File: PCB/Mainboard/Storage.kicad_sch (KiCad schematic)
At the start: 2 parts, among them U41 SDBL-4, U42 SC414281PU4

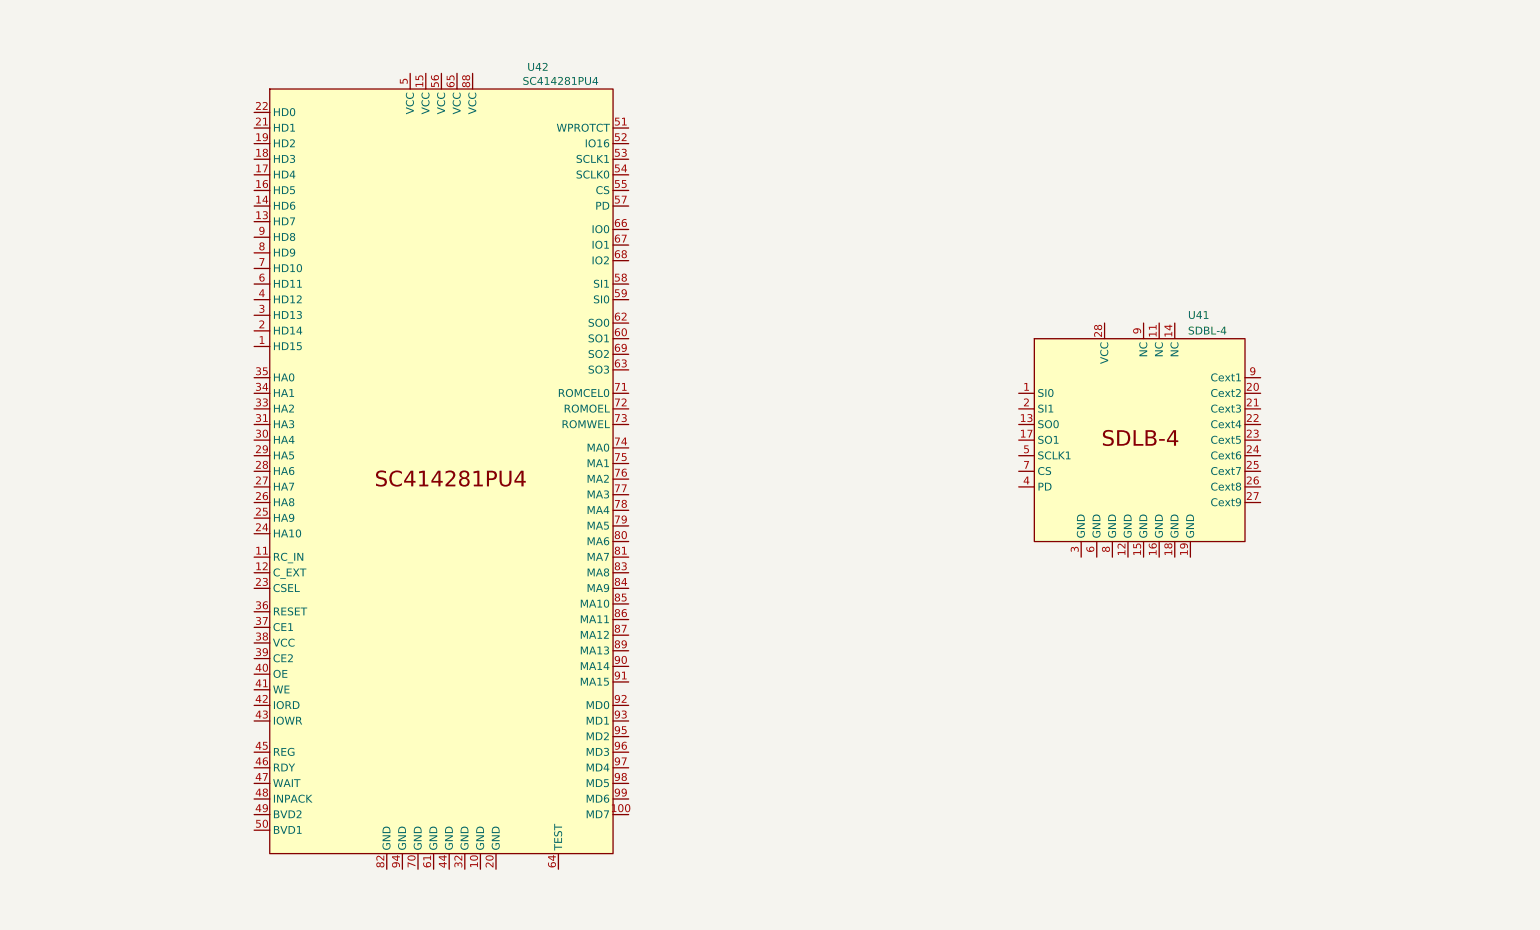
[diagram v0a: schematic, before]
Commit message: Add files via upload
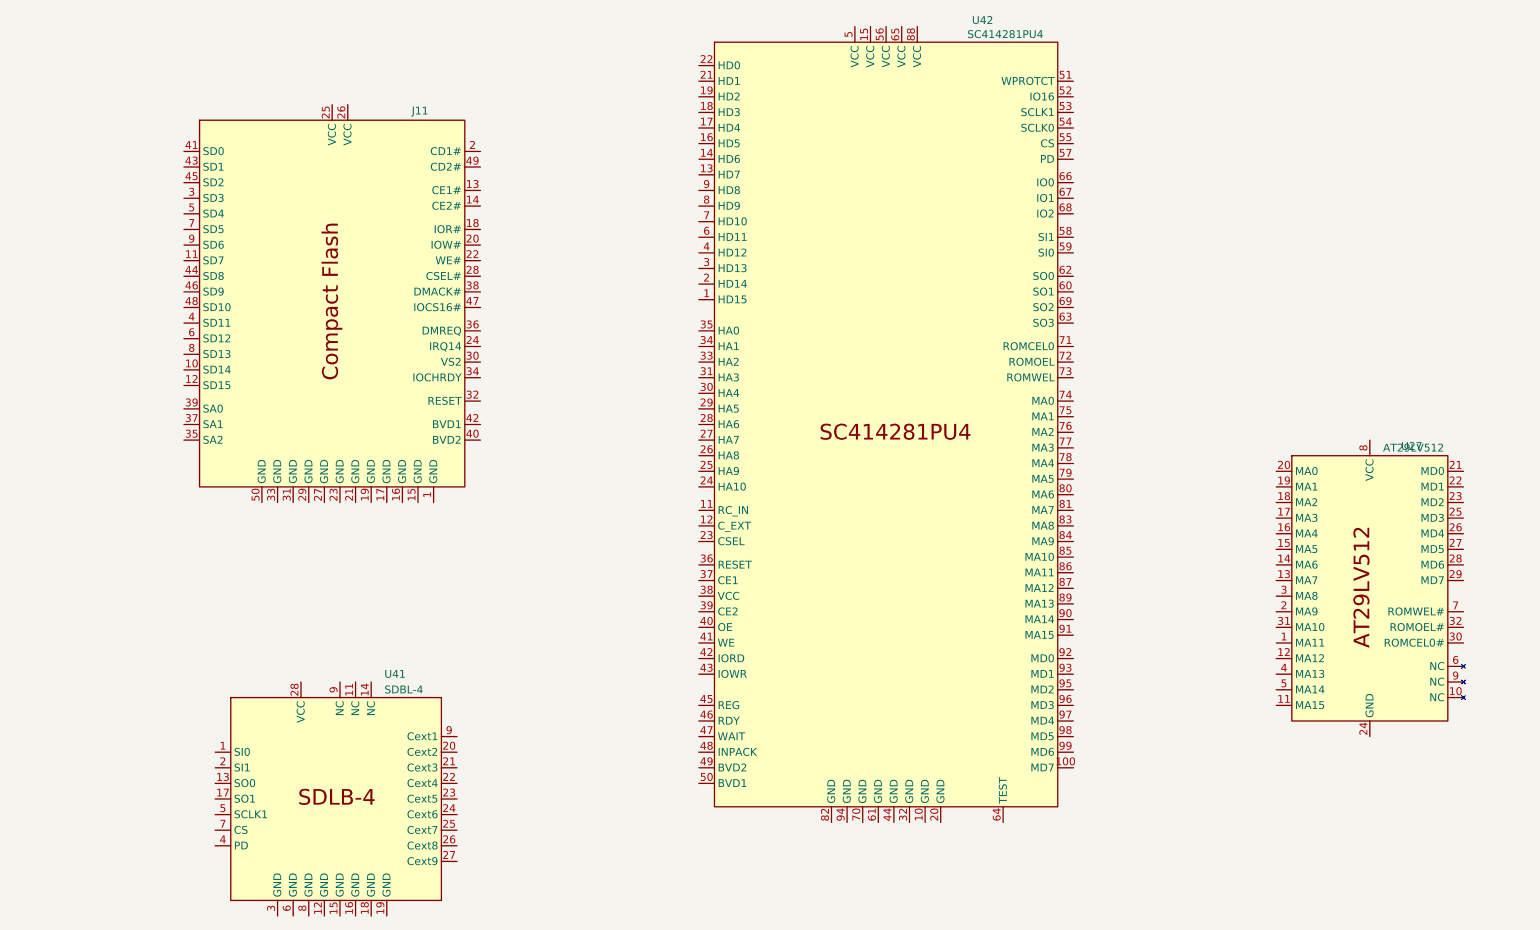
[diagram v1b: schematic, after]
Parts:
- added J11: ~, symbol PC110:CF_Conn
- added U27: AT29LV512, symbol PC110:AT29LV512
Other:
- moved on the sheet: U41, U42

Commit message: Add files via upload
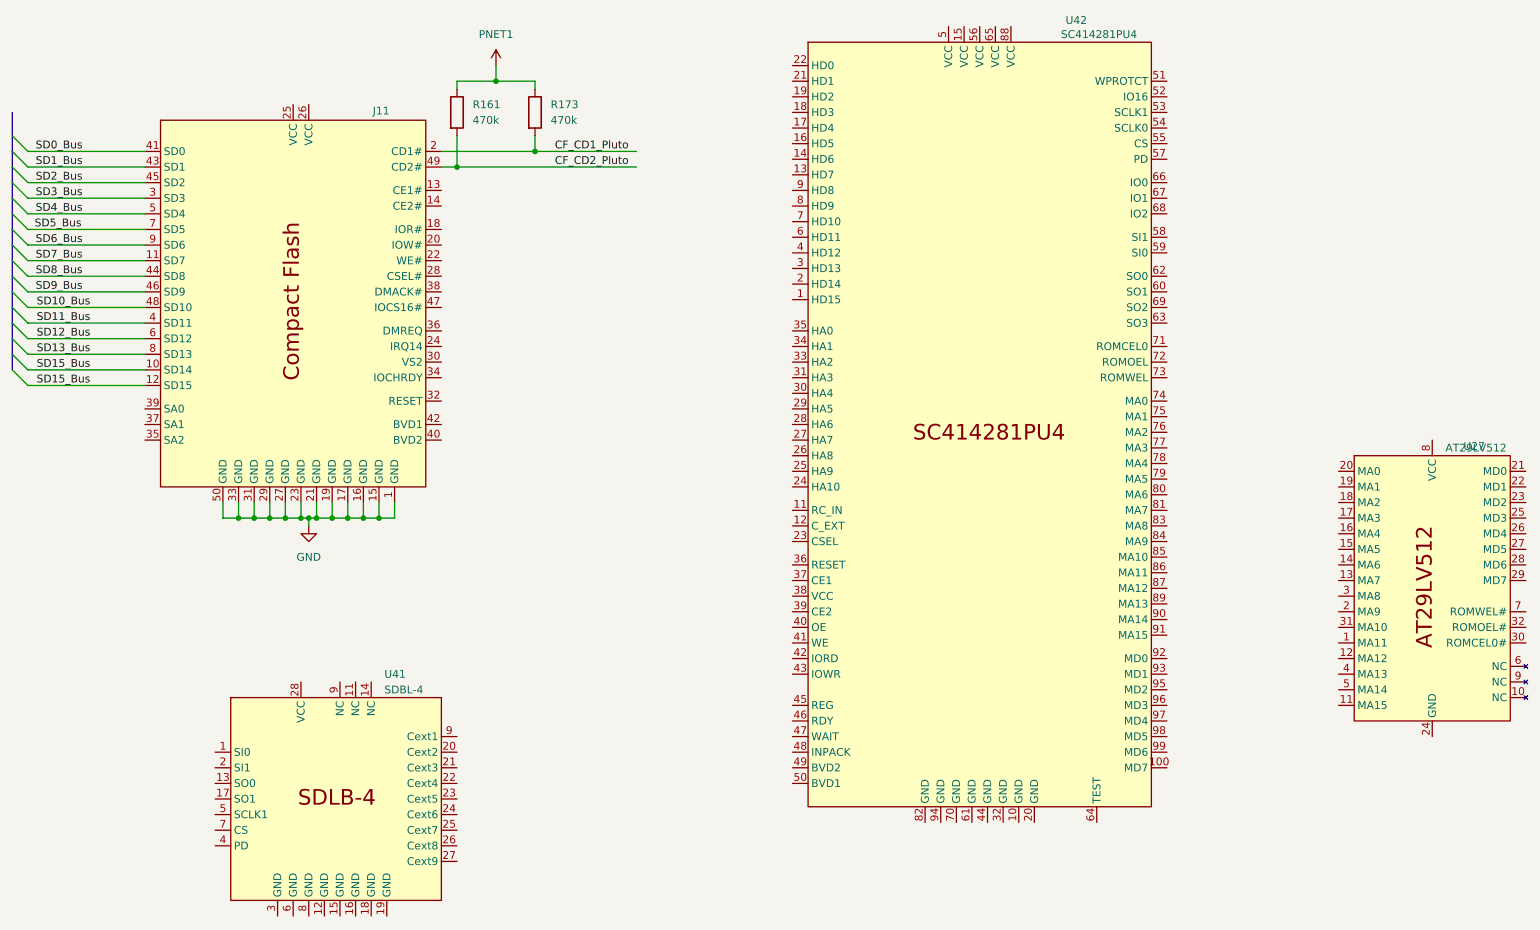
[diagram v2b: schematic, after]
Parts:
- added R161, R173: 470k, symbol Device:R
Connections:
- net GND: now reaches J11.1 (GND)
- net GND: now also J11.15 (GND), J11.16 (GND), J11.17 (GND), J11.19 (GND), J11.21 (GND), J11.23 (GND), J11.27 (GND), J11.29 (GND), J11.31 (GND), J11.33 (GND), J11.50 (GND)
- net SD15_Bus: now reaches J11.10 (SD14)
- net SD15_Bus: now also J11.12 (SD15)
- net SD7_Bus: now reaches J11.11 (SD7)
- net CF_CD1_Pluto: now reaches J11.2 (CD1#)
- net CF_CD1_Pluto: now also R173.2
- net SD3_Bus: now reaches J11.3 (SD3)
- net SD11_Bus: now reaches J11.4 (SD11)
- net SD0_Bus: now reaches J11.41 (SD0)
- net SD1_Bus: now reaches J11.43 (SD1)
- net SD8_Bus: now reaches J11.44 (SD8)
- net SD2_Bus: now reaches J11.45 (SD2)
- net SD9_Bus: now reaches J11.46 (SD9)
- net SD10_Bus: now reaches J11.48 (SD10)
- net CF_CD2_Pluto: now reaches J11.49 (CD2#)
- net CF_CD2_Pluto: now also R161.2
- net SD4_Bus: now reaches J11.5 (SD4)
- net SD12_Bus: now reaches J11.6 (SD12)
- net SD5_Bus: now reaches J11.7 (SD5)
- net SD13_Bus: now reaches J11.8 (SD13)
- net SD6_Bus: now reaches J11.9 (SD6)
- new net PNET1: R161.1, R173.1
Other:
- moved on the sheet: J11, U27, U42
